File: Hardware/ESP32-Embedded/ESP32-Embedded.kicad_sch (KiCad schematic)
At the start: 20 parts, among them J1 10103592-0001LF, Q1 S8050, Q2 S8050, U1 ESP32-WROOM-32E, U2 AMS1117-3.3, U3 CH340G

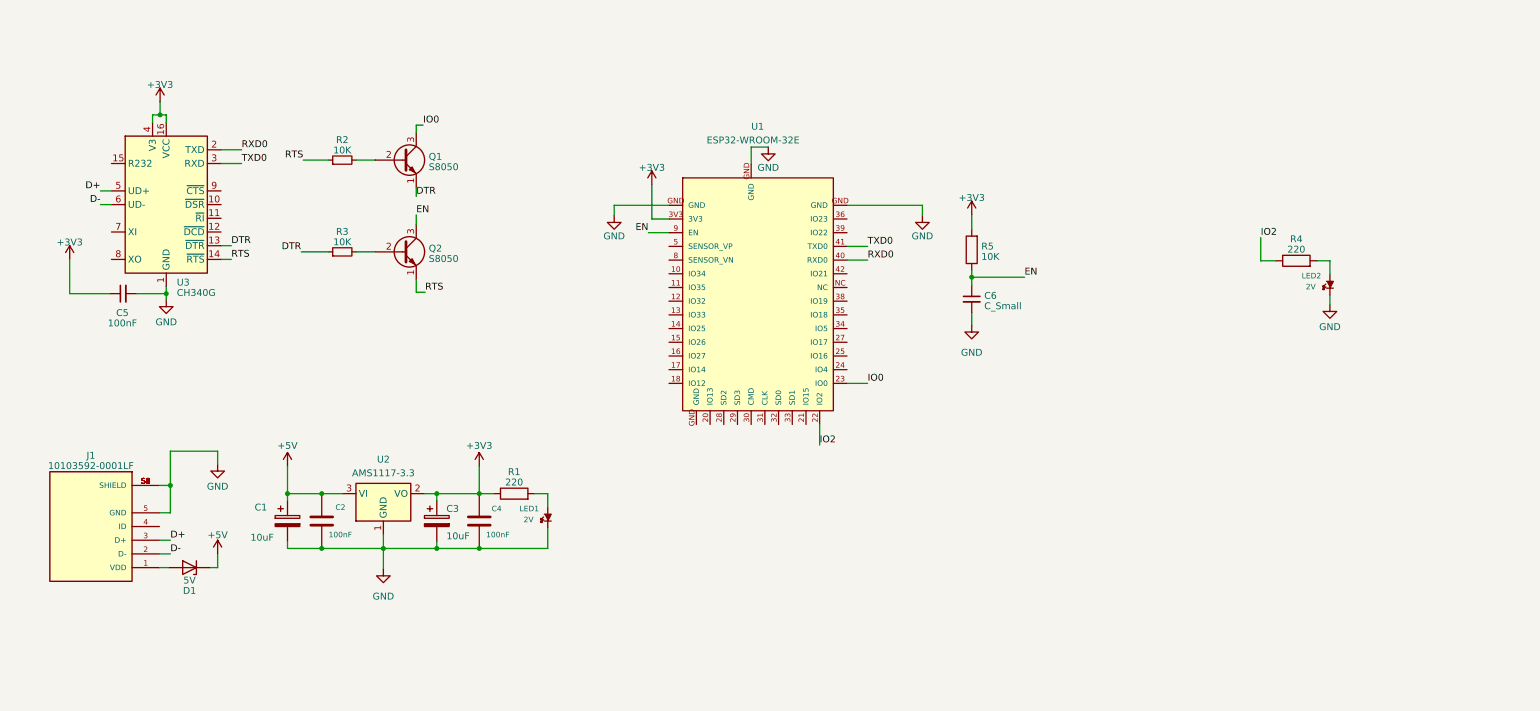
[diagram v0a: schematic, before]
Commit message: sch casi terminado ordene y agregue pocas cosas
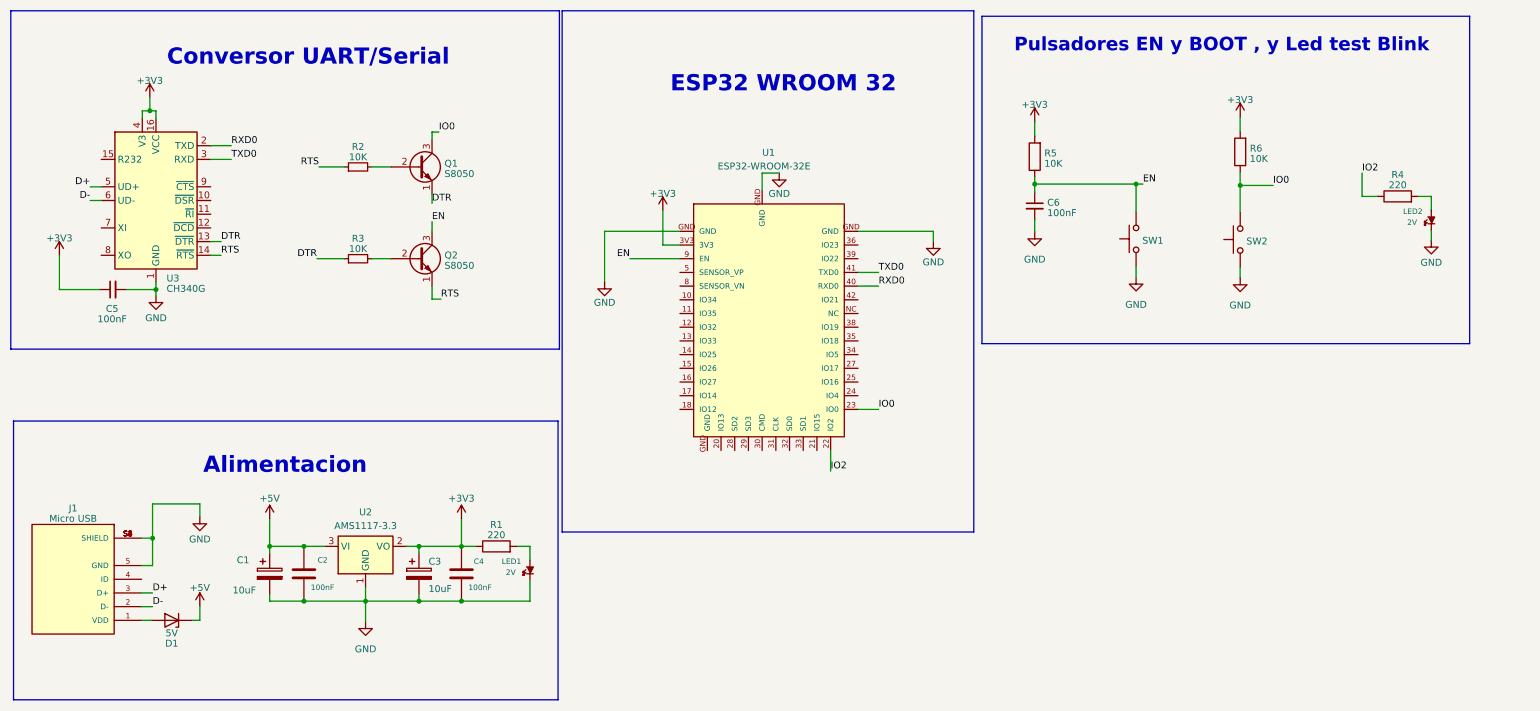
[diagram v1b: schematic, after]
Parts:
- added R6: 10K, EESTN5:R_1206, symbol Device:R
- added SW1, SW2: SW_Push, symbol EESTN5:SW_Push
- C6: value C_Small -> 100nF
- J1: value 10103592-0001LF -> Micro USB
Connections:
- net +3V3: now also R6.2
- net EN: now also SW1.2
- net GND: now also SW1.1, SW2.1
- net IO0: now also R6.1, SW2.2
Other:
- note added: "Alimentacion"
- note added: "Conversor UART/Serial"
- note added: "ESP32 WROOM 32"
- note added: "Pulsadores EN y BOOT , y Led test Blink"
- moved on the sheet: C1, C2, C3, C4, C5, C6, D1, J1, LED1, LED2, Q1, Q2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
